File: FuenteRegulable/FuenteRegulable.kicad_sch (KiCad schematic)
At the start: 56 parts, among them J1 AC_IN, J2 OUT-P, J3 OUT-N, J4 OLED_I2C, Q1 IRF540N, Q2 2N3904, Q3 2N7000, Q4 IRF540N, Q5 2N3904, SW1 SW_MEC_5E, SW2 SW_MEC_5E, SW3 SW_MEC_5E, SW4 SW_MEC_5E, SW5 SW_MEC_5E, SW6 SW_MEC_5E, U2 LM2576T-5, U3 AMS1117-3.3, U4 TL082

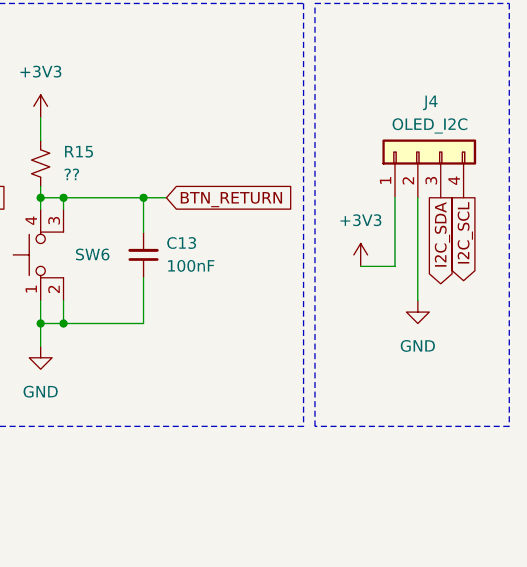
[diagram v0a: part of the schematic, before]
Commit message: Comienzo a rutear PCB
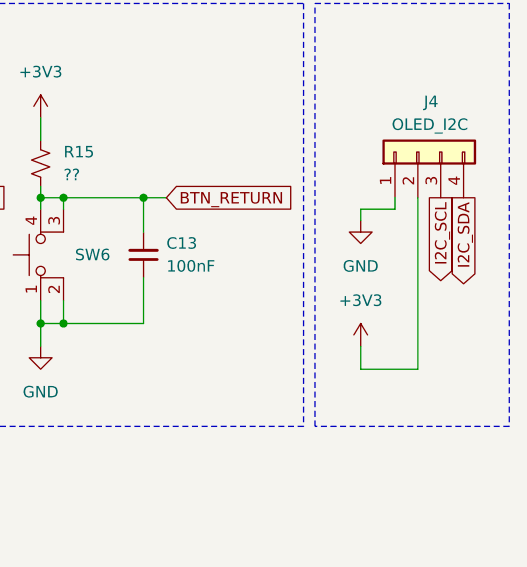
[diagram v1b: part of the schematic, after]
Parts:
- D5, D6: footprint Package_TO_SOT_THT:TO-220-3_Vertical -> Package_TO_SOT_THT:TO-220-3_Horizontal_TabDown
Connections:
- net +3V3: now also J4.2 (Pin_2); no longer J4.1 (Pin_1)
- net GND: now also J4.1 (Pin_1); no longer J4.2 (Pin_2)
- net I2C_SCL: now also J4.3 (Pin_3); no longer J4.4 (Pin_4)
- net I2C_SDA: now also J4.4 (Pin_4); no longer J4.3 (Pin_3)
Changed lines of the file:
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@@
 	)
 	(no_connect
+		(at 43.18 118.11)
+	)
+	(no_connect
 		(at 60.96 123.19)
 	)
@@
 	)
 	(no_connect
-		(at 43.18 118.11)
-	)
-	(no_connect
 		(at 30.48 135.89)
 	)
@@
 	(wire
 		(pts
-			(xy 273.05 138.43) (xy 273.05 127)
+			(xy 273.05 127) (xy 273.05 146.05)
 		)
 		(stroke
@@
 	(wire
 		(pts
-			(xy 266.7 134.62) (xy 270.51 134.62)
+			(xy 266.7 128.27) (xy 270.51 128.27)
 		)
 		(stroke
@@
 	(wire
 		(pts
+			(xy 266.7 146.05) (xy 273.05 146.05)
+		)
+		(stroke
+			(width 0)
+			(type default)
+		)
+	)
+	(wire
+		(pts
 			(xy 215.9 43.18) (xy 215.9 48.26)
 		)
@@
 	(wire
 		(pts
+			(xy 266.7 143.51) (xy 266.7 146.05)
+		)
+		(stroke
+			(width 0)
+			(type default)
+		)
+	)
+	(wire
+		(pts
 			(xy 265.43 91.44) (xy 271.78 91.44)
 		)
@@
 	(wire
 		(pts
-			(xy 270.51 134.62) (xy 270.51 127)
+			(xy 270.51 128.27) (xy 270.51 127)
 		)
 		(stroke
@@
 	(wire
 		(pts
+			(xy 266.7 128.27) (xy 266.7 129.54)
+		)
+		(stroke
+			(width 0)
+			(type default)
+		)
+	)
+	(wire
+		(pts
 			(xy 87.63 140.97) (xy 87.63 143.51)
 		)
@@
 		)
 	)
-	(global_label "I2C_SCL"
-		(shape output)
-		(at 278.13 127 270)
-		(fields_autoplaced yes)
-		(effects
-			(font
-				(size 1.27 1.27)
-			)
-			(justify right)
-		)
-		(property "Intersheetrefs" "${INTERSHEET_REFS}"
-			(at 278.13 137.5447 90)
-			(effects
-				(font
-					(size 1.27 1.27)
-				)
-				(justify right)
-				(hide yes)
-			)
-		)
-	)
 	(global_label "Io_MeasP"
 		(shape input)
@@
 		)
 	)
-	(global_label "I2C_SDA"
-		(shape output)
-		(at 275.59 127 270)
+	(global_label "Vo_ADC"
+		(shape input)
+		(at 30.48 125.73 180)
 		(fields_autoplaced yes)
 		(effects
@@
 		)
 		(property "Intersheetrefs" "${INTERSHEET_REFS}"
-			(at 275.59 137.6052 90)
+			(at 20.661 125.73 0)
 			(effects
 				(font
@@
 		)
 	)
-	(global_label "Vo_ADC"
-		(shape input)
-		(at 30.48 125.73 180)
+	(global_label "I2C_SDA"
+		(shape output)
+		(at 60.96 140.97 0)
 		(fields_autoplaced yes)
 		(effects
@@
 				(size 1.27 1.27)
 			)
-			(justify right)
+			(justify left)
 		)
 		(property "Intersheetrefs" "${INTERSHEET_REFS}"
-			(at 20.661 125.73 0)
+			(at 71.5652 140.97 0)
 			(effects
 				(font
 					(size 1.27 1.27)
 				)
-				(justify right)
+				(justify left)
 				(hide yes)
 			)
@@
 	(global_label "I2C_SDA"
 		(shape output)
-		(at 60.96 140.97 0)
+		(at 278.13 127 270)
 		(fields_autoplaced yes)
 		(effects
@@
 				(size 1.27 1.27)
 			)
-			(justify left)
+			(justify right)
 		)
 		(property "Intersheetrefs" "${INTERSHEET_REFS}"
-			(at 71.5652 140.97 0)
+			(at 278.13 137.6052 90)
 			(effects
 				(font
 					(size 1.27 1.27)
 				)
-				(justify left)
+				(justify right)
 				(hide yes)
 			)
@@
 		)
 	)
+	(global_label "I2C_SCL"
+		(shape output)
+		(at 275.59 127 270)
+		(fields_autoplaced yes)
+		(effects
+			(font
+				(size 1.27 1.27)
+			)
+			(justify right)
+		)
+		(property "Intersheetrefs" "${INTERSHEET_REFS}"
+			(at 275.59 137.5447 90)
+			(effects
+				(font
+					(size 1.27 1.27)
+				)
+				(justify right)
+				(hide yes)
+			)
+		)
+	)
 	(global_label "BTN_PLUS"
 		(shape input)
@@
 	(symbol
 		(lib_id "power:GND")
-		(at 273.05 138.43 0)
+		(at 266.7 129.54 0)
 		(unit 1)
 		(exclude_from_sim no)
@@
 		(dnp no)
 		(property "Reference" "#PWR020"
-			(at 273.05 144.78 0)
+			(at 266.7 135.89 0)
 			(effects
 				(font
@@
 		)
 		(property "Value" "GND"
-			(at 273.05 143.51 0)
+			(at 266.7 134.62 0)
 			(effects
 				(font
@@
 		)
 		(property "Footprint" ""
-			(at 273.05 138.43 0)
+			(at 266.7 129.54 0)
 			(effects
 				(font
@@
 		)
 		(property "Datasheet" ""
-			(at 273.05 138.43 0)
+			(at 266.7 129.54 0)
 			(effects
 				(font
@@
 		)
 		(property "Description" "Power symbol creates a global label with name \"GND\" , ground"
-			(at 273.05 138.43 0)
+			(at 266.7 129.54 0)
 			(effects
 				(font
@@
 	)
 	(symbol
-		(lib_id "power:+3V3")
-		(at 266.7 134.62 0)
-		(unit 1)
-		(exclude_from_sim no)
-		(in_bom yes)
-		(on_board yes)
-		(dnp no)
-		(fields_autoplaced yes)
-		(property "Reference" "#PWR019"
-			(at 266.7 138.43 0)
-			(effects
-				(font
-					(size 1.27 1.27)
-				)
-				(hide yes)
-			)
-		)
-		(property "Value" "+3V3"
-			(at 266.7 129.54 0)
-			(effects
-				(font
-					(size 1.27 1.27)
-				)
-			)
-		)
-		(property "Footprint" ""
-			(at 266.7 134.62 0)
-			(effects
-				(font
-					(size 1.27 1.27)
-				)
-				(hide yes)
-			)
-		)
-		(property "Datasheet" ""
-			(at 266.7 134.62 0)
-			(effects
-				(font
-					(size 1.27 1.27)
-				)
-				(hide yes)
-			)
-		)
-		(property "Description" "Power symbol creates a global label with name \"+3V3\""
-			(at 266.7 134.62 0)
-			(effects
-				(font
-					(size 1.27 1.27)
-				)
-				(hide yes)
-			)
-		)
-		(pin "1"
-		)
-		(instances
-			(project "FuenteRegulable"
-				(path "/5147e114-c546-465f-ae8b-30b4dd1b416a"
-					(reference "#PWR019")
-					(unit 1)
-				)
-			)
-		)
-	)
-	(symbol
 		(lib_id "Device:R_Small_US")
 		(at 130.81 39.37 90)
@@
 			)
 		)
-		(property "Footprint" "Package_TO_SOT_THT:TO-220-3_Vertical"
+		(property "Footprint" "Package_TO_SOT_THT:TO-220-3_Horizontal_TabDown"
 			(at 167.64 34.29 0)
 			(effects
@@
 	)
 	(symbol
+		(lib_id "power:+3V3")
+		(at 266.7 143.51 0)
+		(unit 1)
+		(exclude_from_sim no)
+		(in_bom yes)
+		(on_board yes)
+		(dnp no)
+		(fields_autoplaced yes)
+		(property "Reference" "#PWR031"
+			(at 266.7 147.32 0)
+			(effects
+				(font
+					(size 1.27 1.27)
+				)
+				(hide yes)
+			)
+		)
+		(property "Value" "+3V3"
+			(at 266.7 138.43 0)
+			(effects
+				(font
+					(size 1.27 1.27)
+				)
+			)
+		)
+		(property "Footprint" ""
+			(at 266.7 143.51 0)
+			(effects
+				(font
+					(size 1.27 1.27)
+				)
+				(hide yes)
+			)
+		)
+		(property "Datasheet" ""
+			(at 266.7 143.51 0)
+			(effects
+				(font
+					(size 1.27 1.27)
+				)
+				(hide yes)
+			)
+		)
+		(property "Description" "Power symbol creates a global label with name \"+3V3\""
+			(at 266.7 143.51 0)
+			(effects
+				(font
+					(size 1.27 1.27)
+				)
+				(hide yes)
+			)
+		)
+		(pin "1"
+		)
+		(instances
+			(project "FuenteRegulable"
+				(path "/5147e114-c546-465f-ae8b-30b4dd1b416a"
+					(reference "#PWR031")
+					(unit 1)
+				)
+			)
+		)
+	)
+	(symbol
 		(lib_id "Connector_Generic:Conn_01x04")
 		(at 273.05 121.92 90)
@@
 			)
 		)
-		(property "Footprint" "Package_TO_SOT_THT:TO-220-3_Vertical"
+		(property "Footprint" "Package_TO_SOT_THT:TO-220-3_Horizontal_TabDown"
 			(at 121.92 180.34 0)
 			(effects

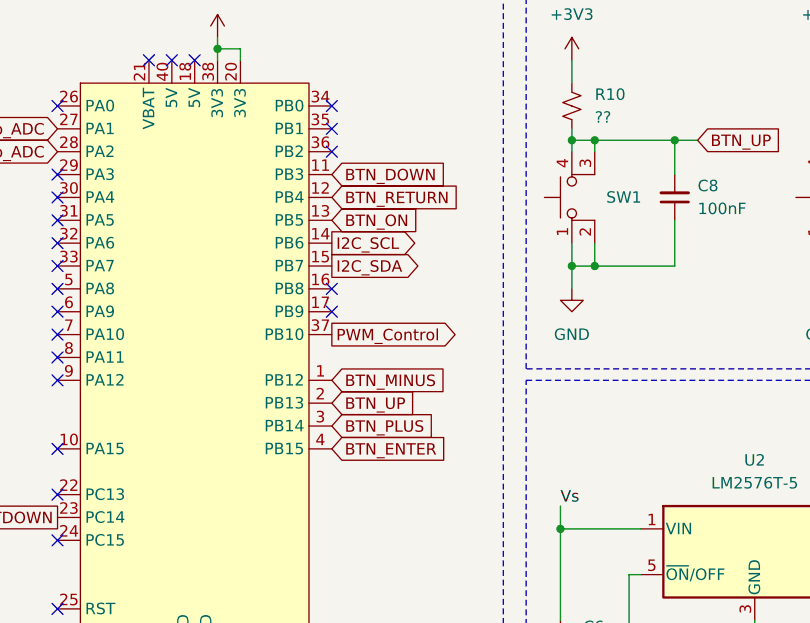
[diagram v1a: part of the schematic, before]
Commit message: PCB Terminado
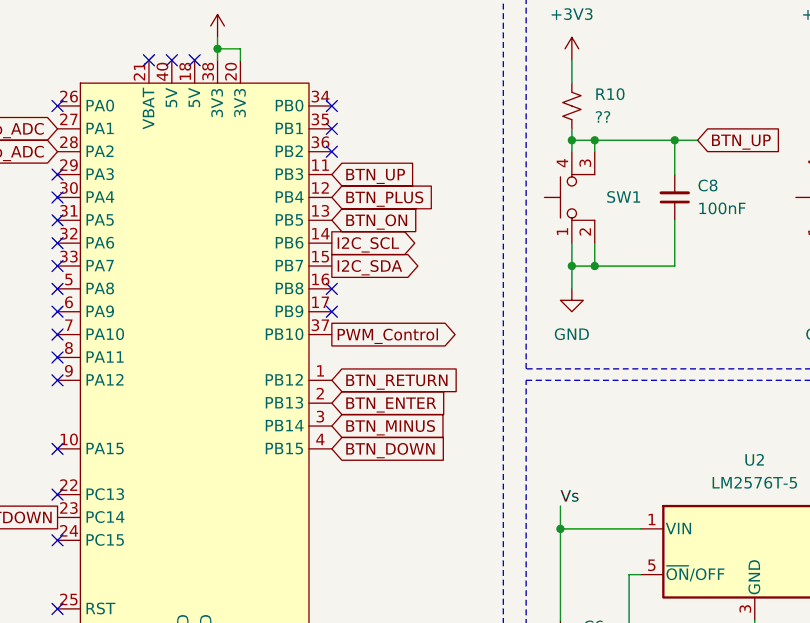
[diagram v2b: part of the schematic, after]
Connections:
- net BTN_DOWN: now also U1.4 (PB15); no longer U1.11 (PB3)
- net BTN_ENTER: now also U1.2 (PB13); no longer U1.4 (PB15)
- net BTN_MINUS: now also U1.3 (PB14); no longer U1.1 (PB12)
- net BTN_PLUS: now also U1.12 (PB4); no longer U1.3 (PB14)
- net BTN_RETURN: now also U1.1 (PB12); no longer U1.12 (PB4)
- net BTN_UP: now also U1.11 (PB3); no longer U1.2 (PB13)
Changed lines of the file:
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@@
-		)
-	)
-	(global_label "BTN_PLUS"
-		(shape input)
-		(at 60.96 158.75 0)
-		(fields_autoplaced yes)
-		(effects
-			(font
-				(size 1.27 1.27)
-			)
-			(justify left)
-		)
-		(property "Intersheetrefs" "${INTERSHEET_REFS}"
-			(at 73.319 158.75 0)
-			(effects
-				(font
-					(size 1.27 1.27)
-				)
-				(justify left)
-				(hide yes)
-			)
 		)
 	)
@@
 		)
 	)
+	(global_label "BTN_RETURN"
+		(shape input)
+		(at 60.96 153.67 0)
+		(fields_autoplaced yes)
+		(effects
+			(font
+				(size 1.27 1.27)
+			)
+			(justify left)
+		)
+		(property "Intersheetrefs" "${INTERSHEET_REFS}"
+			(at 75.7985 153.67 0)
+			(effects
+				(font
+					(size 1.27 1.27)
+				)
+				(justify left)
+				(hide yes)
+			)
+		)
+	)
 	(global_label "Vo_ADC"
 		(shape input)
@@
 		)
 	)
+	(global_label "BTN_ENTER"
+		(shape input)
+		(at 60.96 156.21 0)
+		(fields_autoplaced yes)
+		(effects
+			(font
+				(size 1.27 1.27)
+			)
+			(justify left)
+		)
+		(property "Intersheetrefs" "${INTERSHEET_REFS}"
+			(at 74.347 156.21 0)
+			(effects
+				(font
+					(size 1.27 1.27)
+				)
+				(justify left)
+				(hide yes)
+			)
+		)
+	)
 	(global_label "BTN_DOWN"
 		(shape input)
@@
 		)
 	)
-	(global_label "BTN_RETURN"
-		(shape input)
-		(at 60.96 133.35 0)
-		(fields_autoplaced yes)
-		(effects
-			(font
-				(size 1.27 1.27)
-			)
-			(justify left)
-		)
-		(property "Intersheetrefs" "${INTERSHEET_REFS}"
-			(at 75.7985 133.35 0)
+	(global_label "BTN_UP"
+		(shape input)
+		(at 60.96 130.81 0)
+		(fields_autoplaced yes)
+		(effects
+			(font
+				(size 1.27 1.27)
+			)
+			(justify left)
+		)
+		(property "Intersheetrefs" "${INTERSHEET_REFS}"
+			(at 71.0814 130.81 0)
 			(effects
 				(font
@@
 		)
 	)
-	(global_label "BTN_ENTER"
-		(shape input)
-		(at 60.96 161.29 0)
-		(fields_autoplaced yes)
-		(effects
-			(font
-				(size 1.27 1.27)
-			)
-			(justify left)
-		)
-		(property "Intersheetrefs" "${INTERSHEET_REFS}"
-			(at 74.347 161.29 0)
-			(effects
-				(font
-					(size 1.27 1.27)
-				)
-				(justify left)
-				(hide yes)
-			)
-		)
-	)
 	(global_label "I2C_SCL"
 		(shape output)
@@
 		)
 	)
+	(global_label "Vo_Meas"
+		(shape input)
+		(at 246.38 72.39 180)
+		(fields_autoplaced yes)
+		(effects
+			(font
+				(size 1.27 1.27)
+			)
+			(justify right)
+		)
+		(property "Intersheetrefs" "${INTERSHEET_REFS}"
+			(at 235.4725 72.39 0)
+			(effects
+				(font
+					(size 1.27 1.27)
+				)
+				(justify right)
+				(hide yes)
+			)
+		)
+	)
+	(global_label "BTN_DOWN"
+		(shape input)
+		(at 60.96 161.29 0)
+		(fields_autoplaced yes)
+		(effects
+			(font
+				(size 1.27 1.27)
+			)
+			(justify left)
+		)
+		(property "Intersheetrefs" "${INTERSHEET_REFS}"
+			(at 73.8633 161.29 0)
+			(effects
+				(font
+					(size 1.27 1.27)
+				)
+				(justify left)
+				(hide yes)
+			)
+		)
+	)
+	(global_label "BTN_PLUS"
+		(shape input)
+		(at 60.96 133.35 0)
+		(fields_autoplaced yes)
+		(effects
+			(font
+				(size 1.27 1.27)
+			)
+			(justify left)
+		)
+		(property "Intersheetrefs" "${INTERSHEET_REFS}"
+			(at 73.319 133.35 0)
+			(effects
+				(font
+					(size 1.27 1.27)
+				)
+				(justify left)
+				(hide yes)
+			)
+		)
+	)
+	(global_label "PWM_Control"
+		(shape input)
+		(at 118.11 66.04 180)
+		(fields_autoplaced yes)
+		(effects
+			(font
+				(size 1.27 1.27)
+			)
+			(justify right)
+		)
+		(property "Intersheetrefs" "${INTERSHEET_REFS}"
+			(at 103.0903 66.04 0)
+			(effects
+				(font
+					(size 1.27 1.27)
+				)
+				(justify right)
+				(hide yes)
+			)
+		)
+	)
+	(global_label "BTN_RETURN"
+		(shape input)
+		(at 245.11 127 0)
+		(fields_autoplaced yes)
+		(effects
+			(font
+				(size 1.27 1.27)
+			)
+			(justify left)
+		)
+		(property "Intersheetrefs" "${INTERSHEET_REFS}"
+			(at 259.9485 127 0)
+			(effects
+				(font
+					(size 1.27 1.27)
+				)
+				(justify left)
+				(hide yes)
+			)
+		)
+	)
 	(global_label "BTN_MINUS"
 		(shape input)
-		(at 60.96 153.67 0)
-		(fields_autoplaced yes)
-		(effects
-			(font
-				(size 1.27 1.27)
-			)
-			(justify left)
-		)
-		(property "Intersheetrefs" "${INTERSHEET_REFS}"
-			(at 74.4076 153.67 0)
-			(effects
-				(font
-					(size 1.27 1.27)
-				)
-				(justify left)
-				(hide yes)
-			)
-		)
-	)
-	(global_label "Vo_Meas"
-		(shape input)
-		(at 246.38 72.39 180)
-		(fields_autoplaced yes)
-		(effects
-			(font
-				(size 1.27 1.27)
-			)
-			(justify right)
-		)
-		(property "Intersheetrefs" "${INTERSHEET_REFS}"
-			(at 235.4725 72.39 0)
-			(effects
-				(font
-					(size 1.27 1.27)
-				)
-				(justify right)
-				(hide yes)
-			)
-		)
-	)
-	(global_label "PWM_Control"
-		(shape input)
-		(at 118.11 66.04 180)
-		(fields_autoplaced yes)
-		(effects
-			(font
-				(size 1.27 1.27)
-			)
-			(justify right)
-		)
-		(property "Intersheetrefs" "${INTERSHEET_REFS}"
-			(at 103.0903 66.04 0)
-			(effects
-				(font
-					(size 1.27 1.27)
-				)
-				(justify right)
-				(hide yes)
-			)
-		)
-	)
-	(global_label "BTN_RETURN"
-		(shape input)
-		(at 245.11 127 0)
-		(fields_autoplaced yes)
-		(effects
-			(font
-				(size 1.27 1.27)
-			)
-			(justify left)
-		)
-		(property "Intersheetrefs" "${INTERSHEET_REFS}"
-			(at 259.9485 127 0)
-			(effects
-				(font
-					(size 1.27 1.27)
-				)
-				(justify left)
-				(hide yes)
-			)
-		)
-	)
-	(global_label "BTN_DOWN"
-		(shape input)
-		(at 60.96 130.81 0)
-		(fields_autoplaced yes)
-		(effects
-			(font
-				(size 1.27 1.27)
-			)
-			(justify left)
-		)
-		(property "Intersheetrefs" "${INTERSHEET_REFS}"
-			(at 73.8633 130.81 0)
+		(at 60.96 158.75 0)
+		(fields_autoplaced yes)
+		(effects
+			(font
+				(size 1.27 1.27)
+			)
+			(justify left)
+		)
+		(property "Intersheetrefs" "${INTERSHEET_REFS}"
+			(at 74.4076 158.75 0)
 			(effects
 				(font
@@
 			(effects
 				(font
-					(size 1.27 1.27)
-				)
-				(justify left)
-				(hide yes)
-			)
-		)
-	)
-	(global_label "BTN_UP"
-		(shape input)
-		(at 60.96 156.21 0)
-		(fields_autoplaced yes)
-		(effects
-			(font
-				(size 1.27 1.27)
-			)
-			(justify left)
-		)
-		(property "Intersheetrefs" "${INTERSHEET_REFS}"
-			(at 71.0814 156.21 0)
-			(effects
-				(font
